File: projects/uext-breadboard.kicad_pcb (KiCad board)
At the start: 2 copper layers, 8 parts, among them CON1 UEXT-5V, CON2 UEXT-BREADBOARD, CON3 UEXT-5V, U1 LM1117-3.3

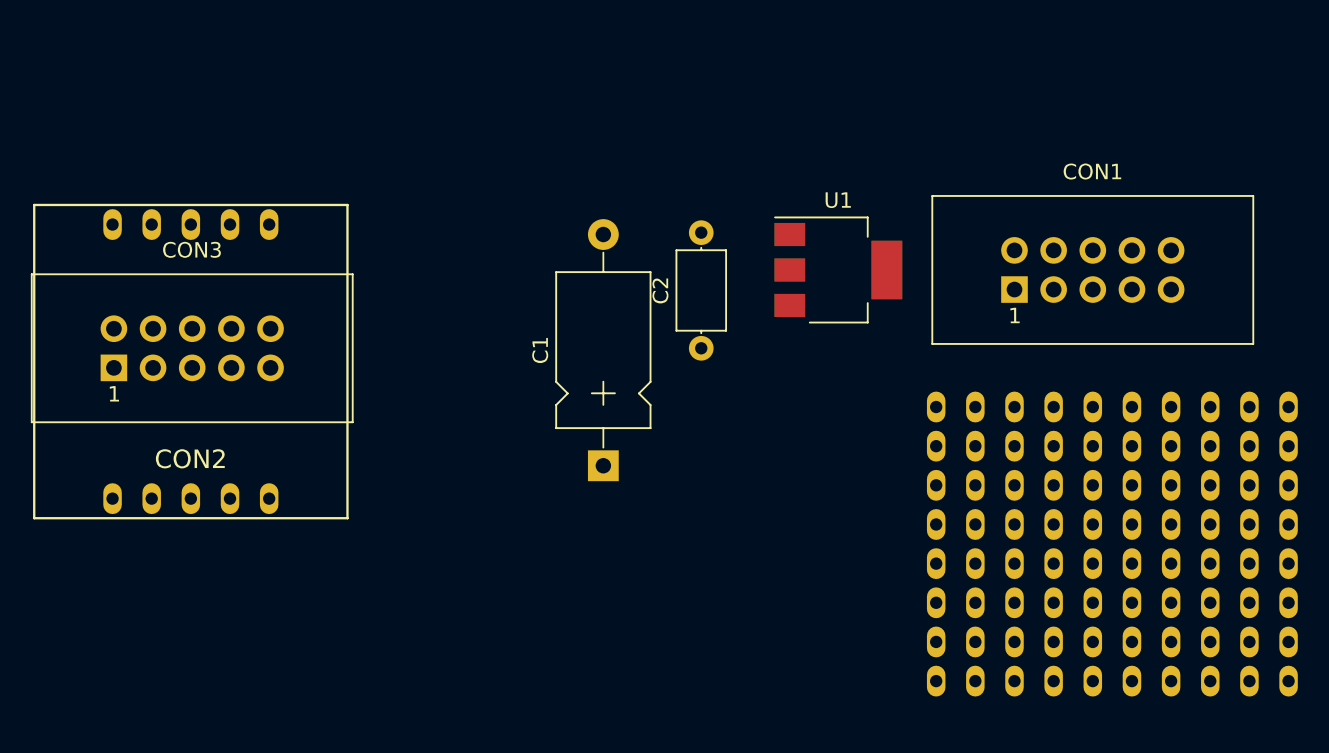
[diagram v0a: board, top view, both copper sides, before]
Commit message: added latest projects
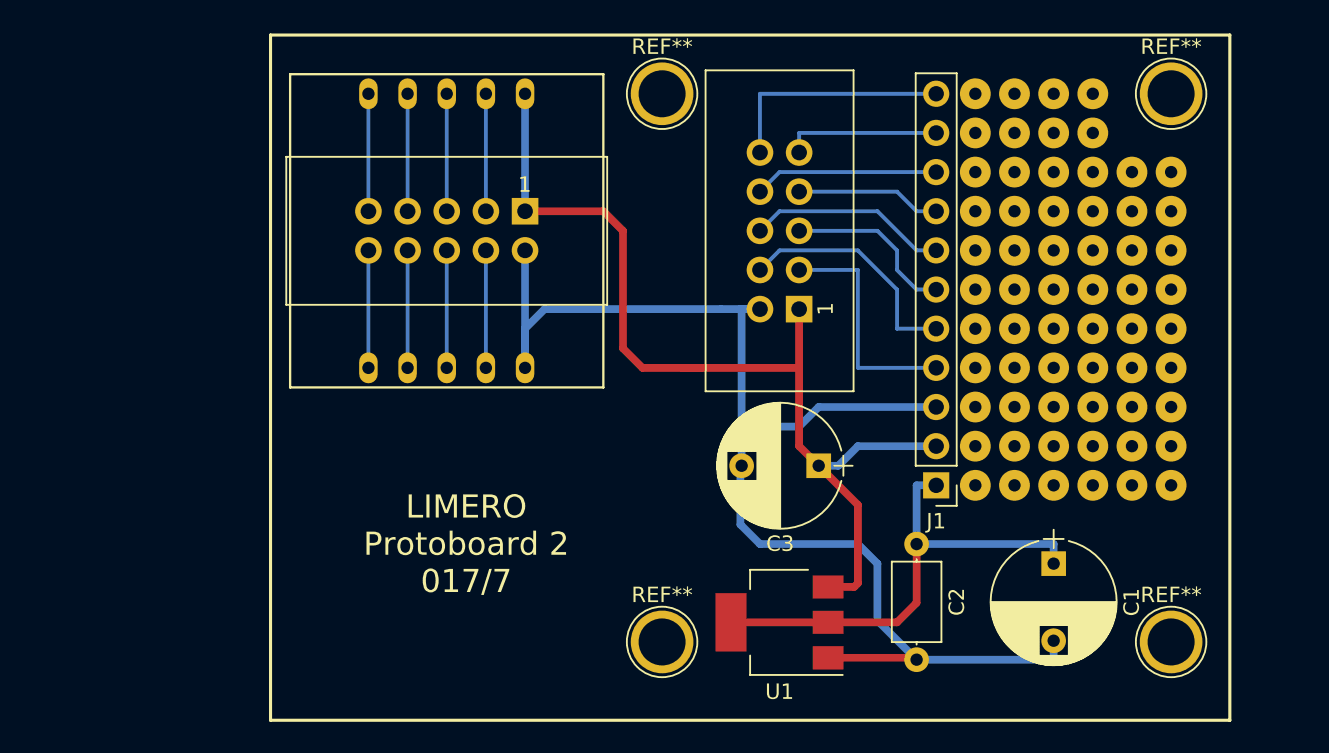
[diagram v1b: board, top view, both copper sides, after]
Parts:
- removed the ? at (199.4, 104.1)
- removed the ? at (199.4, 114.3)
- removed CON1, CON3: UEXT-5V, limero-lib:UEXT
- removed CON2: UEXT-BREADBOARD, limero-lib:UEXT-BREADBOARD
- added ?: , Wire_Pads:SolderWirePad_single_0-8mmDrill, F.Cu at (203.2, 108.0)
- added ?: , Wire_Pads:SolderWirePad_single_0-8mmDrill, F.Cu at (195.6, 105.4)
- added ?: , Wire_Pads:SolderWirePad_single_0-8mmDrill, F.Cu at (193.0, 105.4)
- added ?: , Wire_Pads:SolderWirePad_single_0-8mmDrill, F.Cu at (190.5, 105.4)
- added ?: , Wire_Pads:SolderWirePad_single_0-8mmDrill, F.Cu at (203.2, 102.9)
- added ?: , Wire_Pads:SolderWirePad_single_0-8mmDrill, F.Cu at (200.7, 102.9)
- added ?: , Wire_Pads:SolderWirePad_single_0-8mmDrill, F.Cu at (198.1, 102.9)
- added ?: , Wire_Pads:SolderWirePad_single_0-8mmDrill, F.Cu at (195.6, 102.9)
- added ?: , Wire_Pads:SolderWirePad_single_0-8mmDrill, F.Cu at (193.0, 102.9)
- added ?: , Wire_Pads:SolderWirePad_single_0-8mmDrill, F.Cu at (190.5, 102.9)
- added ?: , Wire_Pads:SolderWirePad_single_0-8mmDrill, F.Cu at (203.2, 100.3)
- added ?: , Wire_Pads:SolderWirePad_single_0-8mmDrill, F.Cu at (200.7, 108.0)
- added ?: , Wire_Pads:SolderWirePad_single_0-8mmDrill, F.Cu at (200.7, 100.3)
- added ?: , Wire_Pads:SolderWirePad_single_0-8mmDrill, F.Cu at (198.1, 100.3)
- added ?: , Wire_Pads:SolderWirePad_single_0-8mmDrill, F.Cu at (195.6, 100.3)
- added ?: , Wire_Pads:SolderWirePad_single_0-8mmDrill, F.Cu at (193.0, 100.3)
- added ?: , Wire_Pads:SolderWirePad_single_0-8mmDrill, F.Cu at (190.5, 100.3)
- added ?: , Wire_Pads:SolderWirePad_single_0-8mmDrill, F.Cu at (203.2, 97.8)
- added ?: , Wire_Pads:SolderWirePad_single_0-8mmDrill, F.Cu at (200.7, 97.8)
- added ?: , Wire_Pads:SolderWirePad_single_0-8mmDrill, F.Cu at (198.1, 97.8)
- added ?: , Wire_Pads:SolderWirePad_single_0-8mmDrill, F.Cu at (195.6, 97.8)
- added ?: , Wire_Pads:SolderWirePad_single_0-8mmDrill, F.Cu at (193.0, 97.8)
- added ?: , Wire_Pads:SolderWirePad_single_0-8mmDrill, F.Cu at (198.1, 108.0)
- added ?: , Wire_Pads:SolderWirePad_single_0-8mmDrill, F.Cu at (190.5, 97.8)
- added ?: , Wire_Pads:SolderWirePad_single_0-8mmDrill, F.Cu at (203.2, 95.2)
- added ?: , Wire_Pads:SolderWirePad_single_0-8mmDrill, F.Cu at (200.7, 95.2)
- added ?: , Wire_Pads:SolderWirePad_single_0-8mmDrill, F.Cu at (198.1, 95.2)
- added ?: , Wire_Pads:SolderWirePad_single_0-8mmDrill, F.Cu at (195.6, 95.2)
- added ?: , Wire_Pads:SolderWirePad_single_0-8mmDrill, F.Cu at (193.0, 95.2)
- added ?: , Wire_Pads:SolderWirePad_single_0-8mmDrill, F.Cu at (190.5, 95.2)
- added ?: , Wire_Pads:SolderWirePad_single_0-8mmDrill, F.Cu at (203.2, 92.7)
- added ?: , Wire_Pads:SolderWirePad_single_0-8mmDrill, F.Cu at (200.7, 92.7)
- added ?: , Wire_Pads:SolderWirePad_single_0-8mmDrill, F.Cu at (198.1, 92.7)
- added ?: , Wire_Pads:SolderWirePad_single_0-8mmDrill, F.Cu at (195.6, 108.0)
- added ?: , Wire_Pads:SolderWirePad_single_0-8mmDrill, F.Cu at (195.6, 92.7)
- added ?: , Wire_Pads:SolderWirePad_single_0-8mmDrill, F.Cu at (193.0, 92.7)
- added ?: , Wire_Pads:SolderWirePad_single_0-8mmDrill, F.Cu at (190.5, 92.7)
- added ?: , Wire_Pads:SolderWirePad_single_0-8mmDrill, F.Cu at (203.2, 90.2)
- added ?: , Wire_Pads:SolderWirePad_single_0-8mmDrill, F.Cu at (200.7, 90.2)
- added ?: , Wire_Pads:SolderWirePad_single_0-8mmDrill, F.Cu at (198.1, 90.2)
- added ?: , Wire_Pads:SolderWirePad_single_0-8mmDrill, F.Cu at (195.6, 90.2)
- added ?: , Wire_Pads:SolderWirePad_single_0-8mmDrill, F.Cu at (193.0, 90.2)
- added ?: , Wire_Pads:SolderWirePad_single_0-8mmDrill, F.Cu at (190.5, 90.2)
- added ?: , Wire_Pads:SolderWirePad_single_0-8mmDrill, F.Cu at (203.2, 87.6)
- added ?: , Wire_Pads:SolderWirePad_single_0-8mmDrill, F.Cu at (193.0, 108.0)
- added ?: , Wire_Pads:SolderWirePad_single_0-8mmDrill, F.Cu at (200.7, 87.6)
- added ?: , Wire_Pads:SolderWirePad_single_0-8mmDrill, F.Cu at (198.1, 87.6)
- added ?: , Wire_Pads:SolderWirePad_single_0-8mmDrill, F.Cu at (195.6, 87.6)
- added ?: , Wire_Pads:SolderWirePad_single_0-8mmDrill, F.Cu at (193.0, 87.6)
- added ?: , Wire_Pads:SolderWirePad_single_0-8mmDrill, F.Cu at (190.5, 87.6)
- added ?: , Wire_Pads:SolderWirePad_single_0-8mmDrill, F.Cu at (198.1, 85.1)
- added ?: , Wire_Pads:SolderWirePad_single_0-8mmDrill, F.Cu at (195.6, 85.1)
- added ?: , Wire_Pads:SolderWirePad_single_0-8mmDrill, F.Cu at (193.0, 85.1)
- added ?: , Wire_Pads:SolderWirePad_single_0-8mmDrill, F.Cu at (190.5, 85.1)
- added ?: , Wire_Pads:SolderWirePad_single_0-8mmDrill, F.Cu at (198.1, 82.5)
- added ?: , Wire_Pads:SolderWirePad_single_0-8mmDrill, F.Cu at (190.5, 108.0)
- added ?: , Wire_Pads:SolderWirePad_single_0-8mmDrill, F.Cu at (195.6, 82.5)
- added ?: , Wire_Pads:SolderWirePad_single_0-8mmDrill, F.Cu at (193.0, 82.5)
- added ?: , limero-lib:UEXT, F.Cu at (179.1, 96.5)
- added ?: , limero-lib:UEXT-BREADBOARD, F.Cu at (156.2, 91.4)
- added ?: , limero-lib:UEXT, F.Cu at (161.3, 90.2)
- added ?: , Wire_Pads:SolderWirePad_single_0-8mmDrill, F.Cu at (190.5, 82.5)
- added ?: , Wire_Pads:SolderWirePad_single_0-8mmDrill, F.Cu at (203.2, 105.4)
- added ?: , Wire_Pads:SolderWirePad_single_0-8mmDrill, F.Cu at (200.7, 105.4)
- added ?: , Wire_Pads:SolderWirePad_single_0-8mmDrill, F.Cu at (198.1, 105.4)
- added C3: CP, Capacitors_THT:CP_Radial_D8.0mm_P5.00mm, F.Cu at (180.3, 106.7)
- added J1: , Pin_Headers:Pin_Header_Straight_1x11_Pitch2.54mm, F.Cu at (188.0, 108.0)
- added REF**: 1pin, Connectors:1pin, F.Cu at (170.2, 118.1)
- added REF**: 1pin, Connectors:1pin, F.Cu at (170.2, 82.5)
- added REF**: 1pin, Connectors:1pin, F.Cu at (203.2, 82.5)
- added REF**: 1pin, Connectors:1pin, F.Cu at (203.2, 118.1)
- C1: footprint Capacitors_THT:CP_Axial_L10.0mm_D6.0mm_P15.00mm_Horizontal -> Capacitors_THT:CP_Radial_D8.0mm_P5.00mm
- moved C1 29.9 mm to (195.6, 113.0), turned to 270 degrees
- moved U1 23.2 mm to (177.8, 116.8), turned to 180 degrees
- moved C2 18.9 mm to (186.7, 111.8), turned to 270 degrees
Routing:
- net GND: track 0.00 -> 87.4 mm
- net +5V: track 0.00 -> 64.9 mm
- net +3V3: track 0.00 -> 31.6 mm
- net RXD: track 0.00 -> 15.5 mm
- net TXD: track 0.00 -> 15.2 mm
- net SSEL: track 0.00 -> 15.2 mm
- net SDA: track 0.00 -> 13.0 mm
- net MOSI: track 0.00 -> 12.0 mm
- net SCL: track 0.00 -> 11.2 mm
- net SCK: track 0.00 -> 10.2 mm
- net MISO: track 0.00 -> 9.42 mm
- net Net-(CON2-PadTXD): track 0.00 -> 7.62 mm
- net Net-(CON2-PadSSEL): track 0.00 -> 7.62 mm
- net Net-(CON2-PadSDA): track 0.00 -> 7.62 mm
- net Net-(CON2-PadSCL): track 0.00 -> 7.62 mm
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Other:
- net class power added: clearance 0.2, trace_width 0.5, via_dia 0.6, via_drill 0.4
- board text added: "LIMERO Protoboard 2 017/7"
